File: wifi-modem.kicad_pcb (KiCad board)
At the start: 2 copper layers, 68.6 x 74 mm, 47 parts, among them J1 RS232, J2 USB Power, SW1 RESET, SW2 PROG, U1 ESP-12F, U2 MAX3238EAIT, U3 AMS1117-3.3

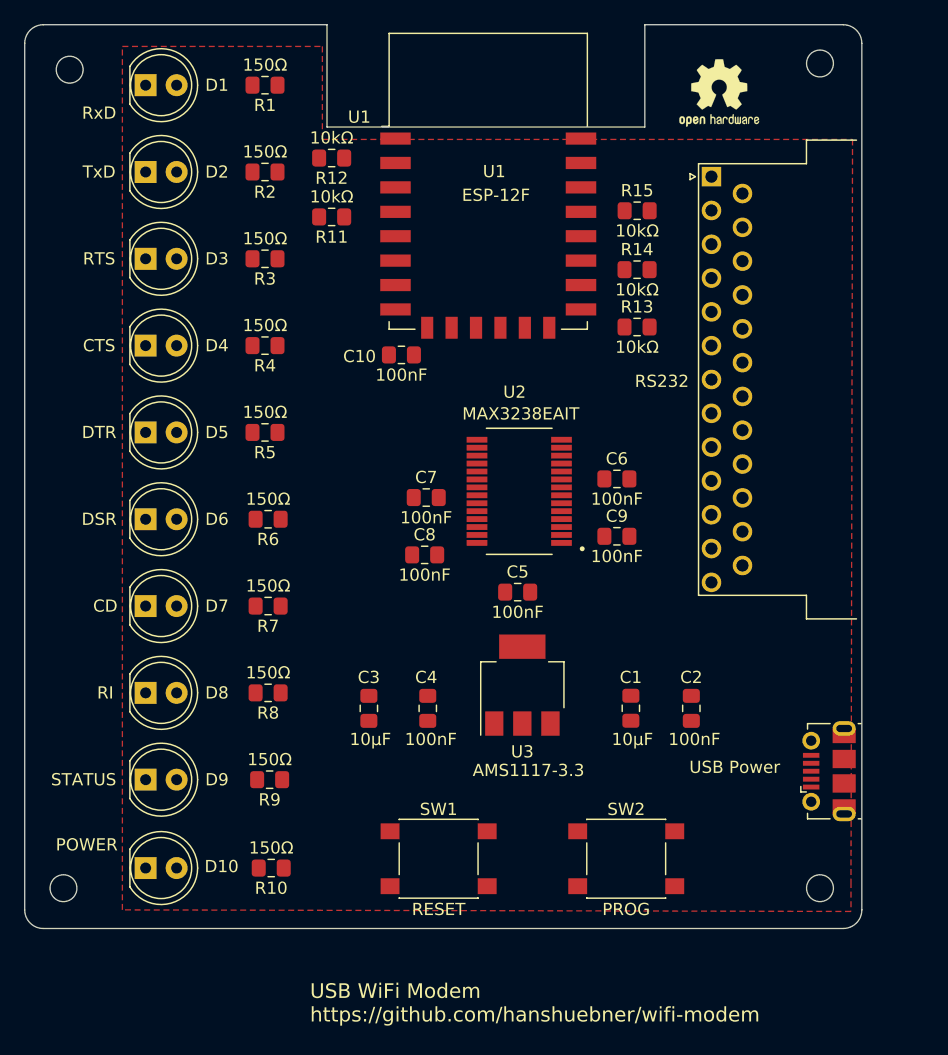
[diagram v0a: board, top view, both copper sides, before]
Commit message: Layout redone
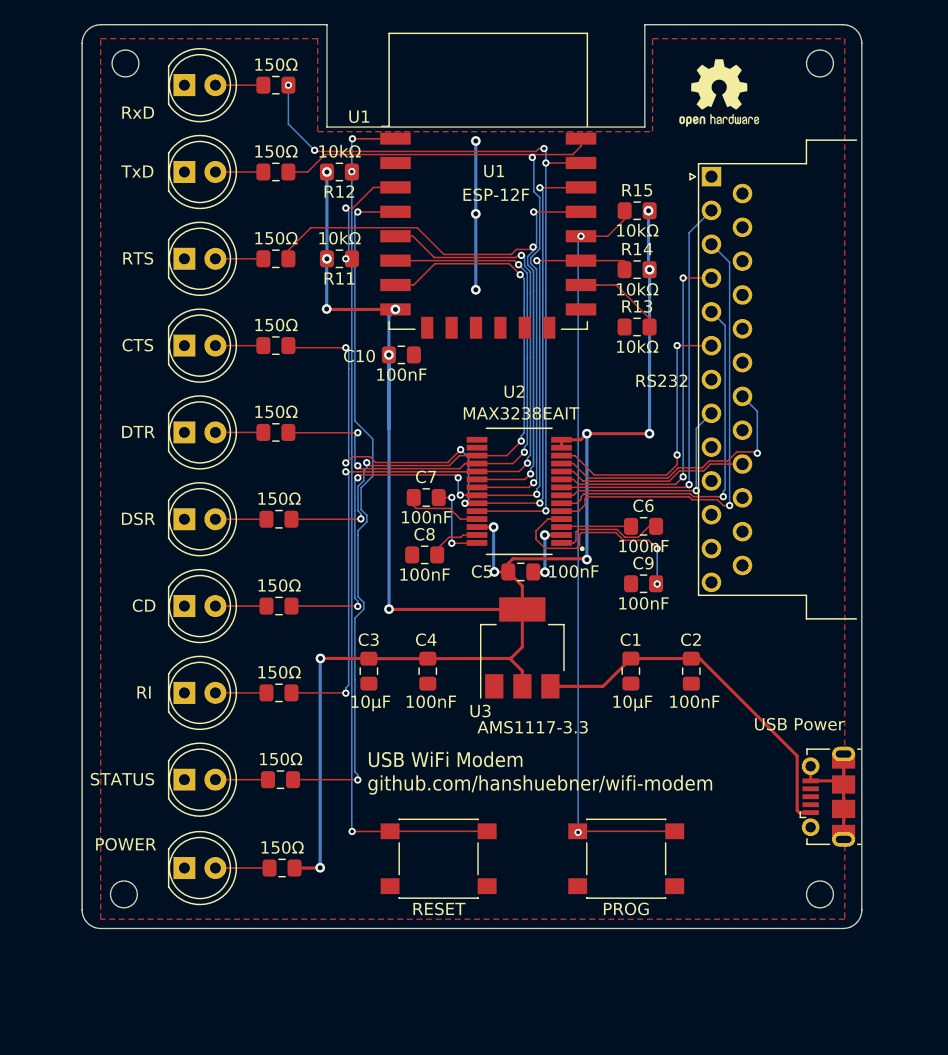
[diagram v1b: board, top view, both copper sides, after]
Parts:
- moved REF** 4.98 mm to (118.7, 134.6)
- moved REF** 4.60 mm to (118.9, 66.5)
- moved C6 4.46 mm to (161.3, 104.5)
- moved C9 4.46 mm to (161.3, 109.2)
- moved R11 3.49 mm to (136.4, 82.5)
- moved D1 3.17 mm to (123.7, 68.3)
- moved D10 3.17 mm to (123.7, 132.5)
- moved D2 3.17 mm to (123.7, 75.4)
- moved D3 3.17 mm to (123.7, 82.5)
- moved D4 3.17 mm to (123.7, 89.7)
- moved D5 3.17 mm to (123.7, 96.8)
- moved D6 3.17 mm to (123.7, 103.9)
- moved D7 3.17 mm to (123.7, 111.0)
- moved D8 3.17 mm to (123.7, 118.1)
- moved D9 3.17 mm to (123.7, 125.2)
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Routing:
- net +3V3: track 0.00 -> 154.5 mm, vias 0 -> 15
- net /~RST: track 0.00 -> 71.4 mm, vias 0 -> 3
- net /RI: track 0.00 -> 66.7 mm, vias 0 -> 4
- net /CTS: track 0.00 -> 65.1 mm, vias 0 -> 6
- net /RxD: track 0.00 -> 63.4 mm, vias 0 -> 5
- net Net-(R15-Pad1): track 0.00 -> 61.8 mm, vias 0 -> 2
- net /CD: track 0.00 -> 59.6 mm, vias 0 -> 6
- net /TxD: track 0.00 -> 58.8 mm, vias 0 -> 2
- net Net-(R9-Pad1): track 0.00 -> 57.1 mm, vias 0 -> 2
- net /RTS: track 0.00 -> 53.3 mm, vias 0 -> 3
- net /DSR: track 0.00 -> 49.5 mm, vias 0 -> 4
- net /DTR: track 0.00 -> 49.0 mm, vias 0 -> 4
- net Net-(J1-Pad3): track 0.00 -> 36.9 mm, vias 0 -> 1
- net Net-(J1-Pad2): track 0.00 -> 33.8 mm, vias 0 -> 1
- net Net-(C1-Pad1): track 0.00 -> 30.1 mm
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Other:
- board size 68.6 x 74 mm -> 63.9 x 74 mm
- board text added: "USB WiFi Modem github.com/hanshuebner/wifi-modem"
- board text removed: "USB WiFi Modem https://github.com/hanshuebner/wifi-modem"
